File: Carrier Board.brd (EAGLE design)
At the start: 88 x 34.9 mm, 57 parts, among them J4 S2B-PH-SM4-TB(LF)(SN), J5 S2B-PH-SM4-TB(LF)(SN), Q1 MMBT2222A, U1 TMP36GRTZ, U2 TPL5010, U3 MB85RC256, U4 Particle Electron, U5 TPS22810, U6 TPS22810, U7 NAND

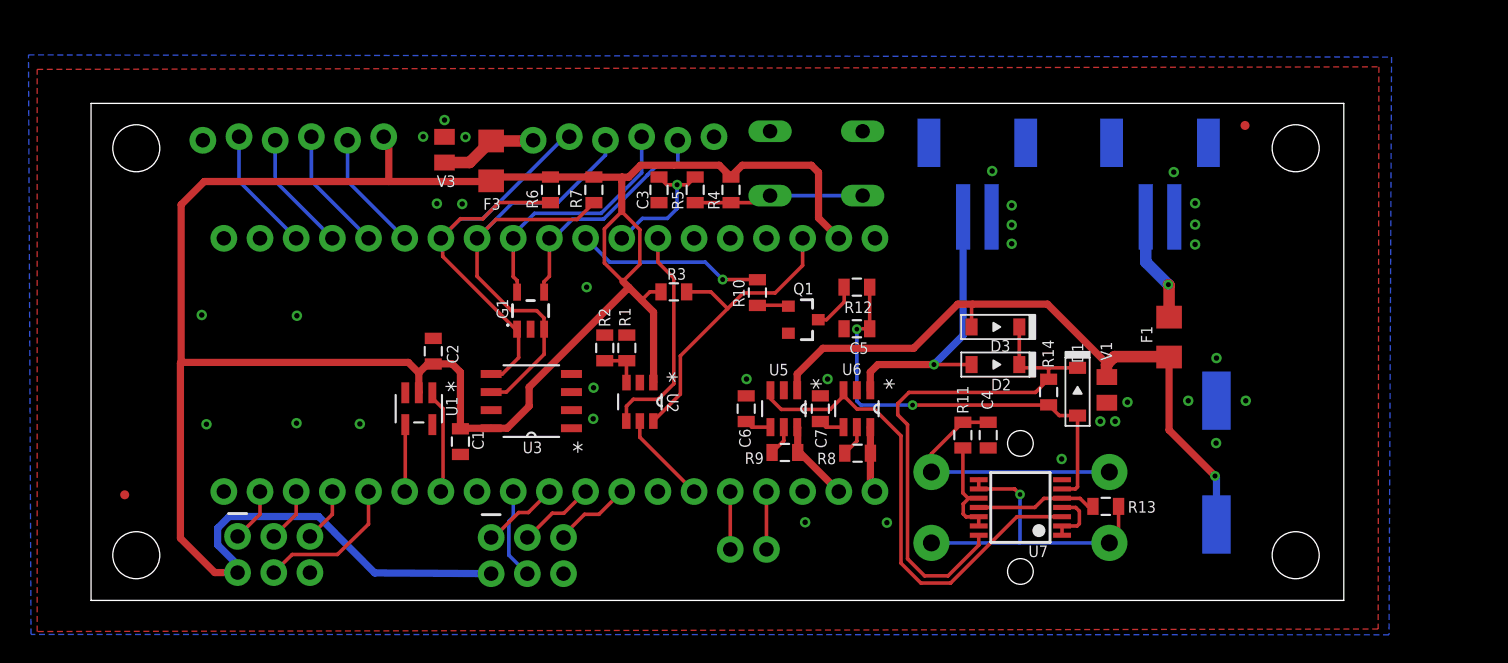
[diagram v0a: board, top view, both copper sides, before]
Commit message: v0.1 - First rough layout
Just getting started.
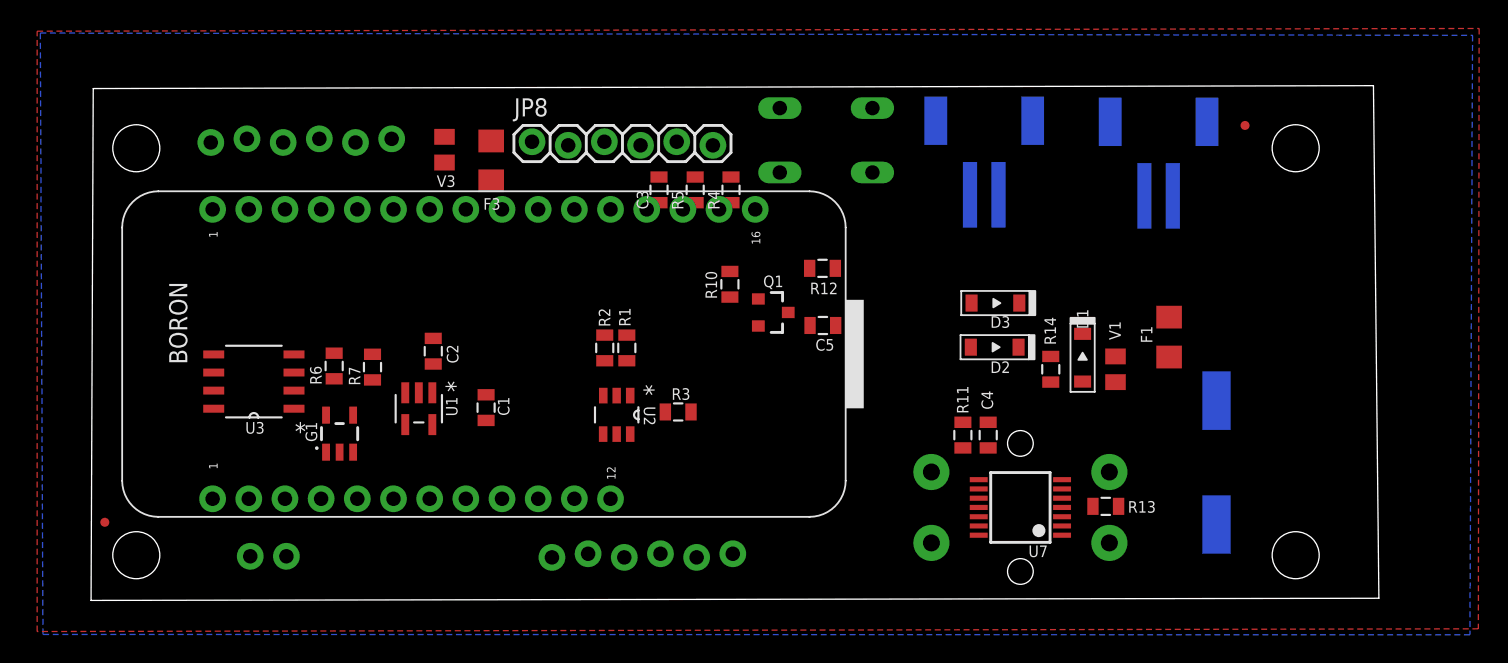
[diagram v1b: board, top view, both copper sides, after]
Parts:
- removed C6, C7: 0.1uF, SparkFun-Capacitors:0805@1
- removed J1, J2/SPI: (no value), SparkFun-Connectors:2X3
- removed R8, R9: 100, SparkFun-Passives:0805
- removed U4: Particle Electron, Particle-Devices:ELECTON-PWR-PINS
- removed U5, U6: TPS22810, Custom Components:SOT-23-6
- added BORON: PARTICLE-DEVICES-BORON, Carrier Board:PARTICLE-DEVICES_BORON
- added JP8: (no value), SparkFun-Connectors:1X06_LOCK
- moved J3 31.2 mm to (13.7, 3.10), turned to 0 degrees
- moved JP1 29.3 mm to (45.1, 3.28)
- moved R7 19.9 mm to (19.8, 16.4)
- moved R6 19.6 mm to (17.1, 16.5)
- moved U3 19.5 mm to (11.4, 15.4)
- moved G1 16.0 mm to (17.4, 11.7)
- moved R3 8.44 mm to (41.2, 13.2)
- moved C1 2.99 mm to (27.7, 13.5)
- moved R12 2.75 mm to (51.4, 23.3)
- moved D1 2.41 mm to (69.6, 17.0)
- moved C5 2.40 mm to (51.4, 19.3)
- moved FD2 2.38 mm to (0.97, 5.49)
- moved Q1 2.17 mm to (47.9, 20.2)
- moved R10 2.02 mm to (44.9, 22.2)
- moved U2 1.87 mm to (36.9, 13.0)
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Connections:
- removed net A4: J2/SPI.3, U4.8
- removed net B0: U4.18
- removed net B1: J1.1, U4.17
- removed net B2: J1.3, U4.16
- removed net B3: J1.5, U4.15
- removed net B4: J1.4, U4.14
- removed net BATT-IN: D2.ANODE, J5.2, U6.1
- removed net C0: U4.19
- removed net C1: U4.20
- removed net C2: JP2.2, U4.21
- removed net C3: JP2.3, U4.22
- removed net C4: JP2.4, U4.23
- removed net C5: JP2.5, U4.24
- removed net DAC: U4.6
- removed net DC-IN: C8.P$1, D3.ANODE, F1.2, U5.1, V1.2
- removed net N$2: C6.1, U5.4
- removed net N$5: C7.1, U6.4
- removed net N$6: R8.1, U6.5
- removed net N$7: R9.1, U5.5
- removed net ON/OFF: U5.3, U6.3, U7.3
- removed net VBAT: U4.34
- removed net VIN: R9.2, U4.1, U5.6
- new net 3V3: BORON.3V3
- new net A0: BORON.A0, JP8.5
- new net D7: BORON.D7
- new net EN: BORON.EN, U7.3
- new net MD: BORON.MD
- new net MISO: BORON.MI, JP2.3
- new net MOSI: BORON.MO, JP2.4
- new net SCK: BORON.SCK, JP2.5
- new net VUSB: BORON.VUSB, C8.P$1, D3.ANODE, F1.2, V1.2
- new net WAKE: BORON.D6
- net !RST: now also BORON.RST; no longer U4.35
- net !SHTDWN: now also BORON.D8; no longer U4.13
- net A1: now also BORON.A1, JP8.4; no longer U4.11
- net A2: now also BORON.A2, JP8.3; no longer J2/SPI.4, U4.10
- net A3: now also BORON.A3, JP8.2; no longer J2/SPI.1, U4.9
- net A5: now also BORON.A5, JP2.2; no longer J2/SPI.5, U4.7
- net D2: now also BORON.D2; no longer U4.27
- net D3: now also BORON.D3; no longer U4.28
- net DONE: now also BORON.D5; no longer U4.31
- net GND: now also BORON.GND, JP8.1; no longer C6.2, C7.2, J1.6, J2/SPI.6, U4.2, U4.33, U5.2, U6.2
- net HARD-RESET: no longer U4.29
- net LI+: now also BORON.LI+, D2.ANODE, J5.2; no longer R8.2, U4.LI+, U6.6
- net RX: now also BORON.RX; no longer U4.4
- net SCL: now also BORON.SCL; no longer U4.26
- net SDA: now also BORON.SDA; no longer U4.25
- net TEMP: now also BORON.A4; no longer U4.12
- net TX: now also BORON.TX; no longer U4.3
- net USER-SW: now also BORON.D4; no longer U4.30
- net VCC: now also JP8.6; no longer J1.2, J2/SPI.2, JP2.6, U4.36
- net VCC-EXT: now also JP2.6
- net WKP: no longer U4.5
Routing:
- net VCC: track 175.1 -> 0.00 mm
- net DC-IN: track 47.0 -> 0.00 mm, vias 1 -> 0
- net SCL: track 38.0 -> 0.00 mm
- net ENABLE-PWR: track 37.2 -> 0.00 mm
- net ON/OFF: track 35.2 -> 0.00 mm
- net SDA: track 33.8 -> 0.00 mm
- net !HARD-RESET: track 31.0 -> 0.00 mm, vias 2 -> 0
- net N$25: track 22.5 -> 0.00 mm, vias 1 -> 0
- net !RST: track 21.8 -> 0.00 mm
- net BATT-IN: track 19.8 -> 0.00 mm, vias 1 -> 0
- net N$24: track 18.7 -> 0.00 mm
- net D2: track 17.5 -> 0.00 mm
- net D3: track 16.8 -> 0.00 mm
- net DONE: track 15.7 -> 0.00 mm
- net HARD-RESET: track 13.3 -> 0.00 mm, vias 1 -> 0
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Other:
- board size 88 x 34.9 mm -> 90.4 x 36.1 mm
